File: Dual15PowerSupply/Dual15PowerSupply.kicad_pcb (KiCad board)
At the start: 2 copper layers, 100 x 100 mm, 37 parts, among them J1 120VAC, J2 +/-15VDC, U1 LT3091, U2 LT3081

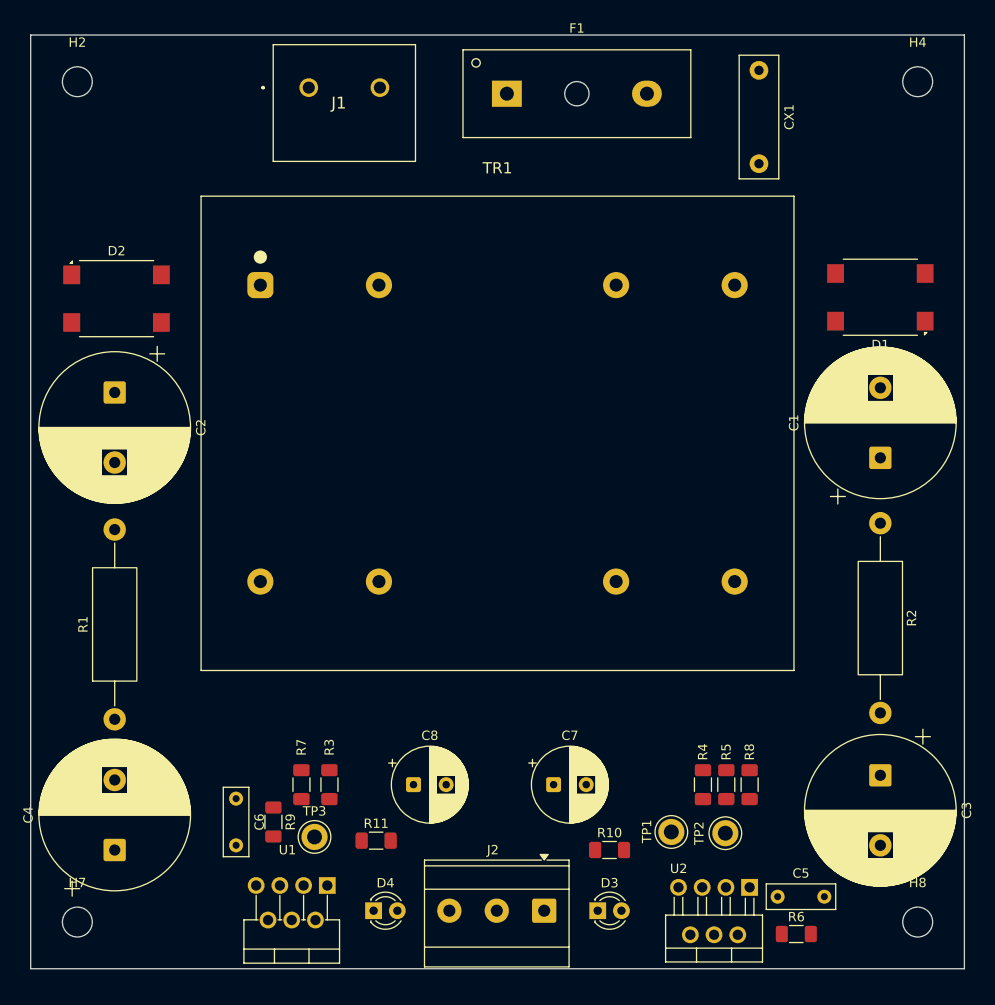
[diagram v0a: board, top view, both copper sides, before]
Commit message: Layout in progress
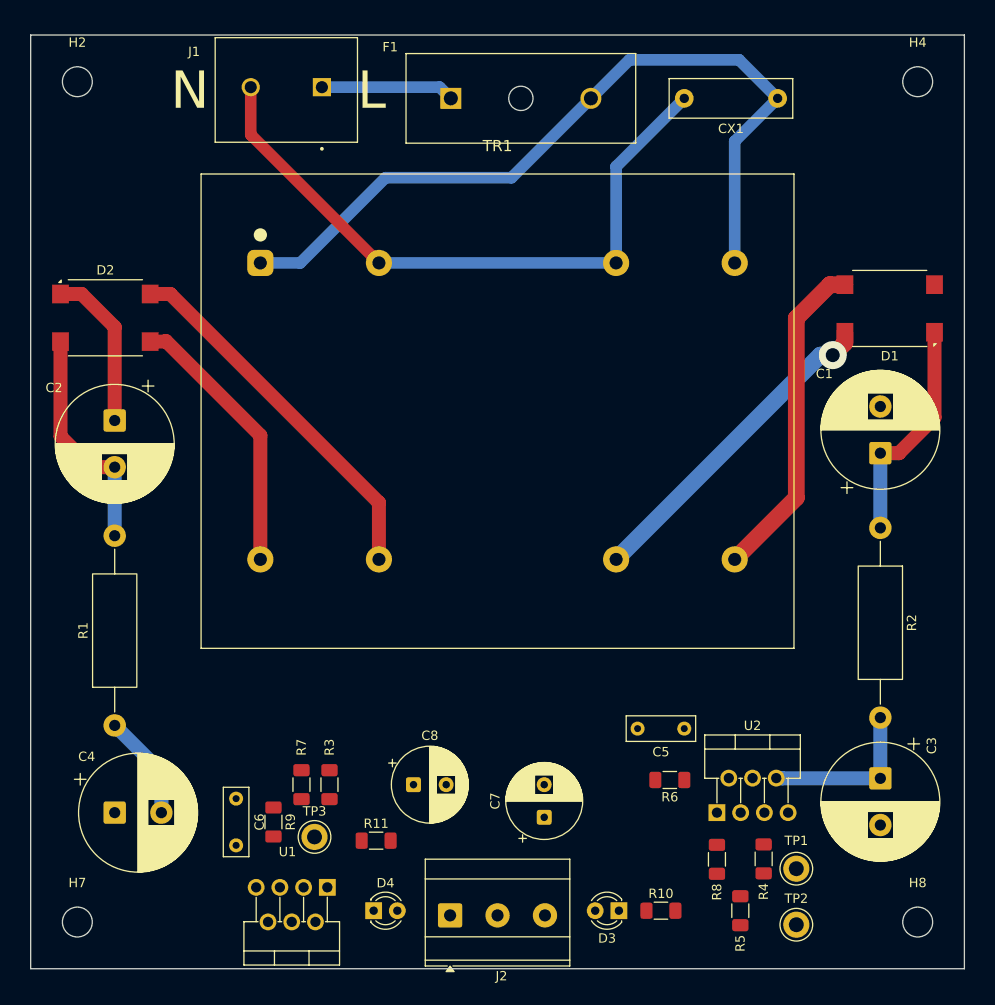
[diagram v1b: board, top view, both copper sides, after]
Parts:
- C1, C2: value 2200µF -> 1000µF; footprint Capacitor_THT:CP_Radial_D16.0mm_P7.50mm -> Capacitor_THT:CP_Radial_D12.5mm_P5.00mm
- C3, C4: footprint Capacitor_THT:CP_Radial_D16.0mm_P7.50mm -> Capacitor_THT:CP_Radial_D12.5mm_P5.00mm
- F1: footprint Fuseholder_Wurth:Wurth_WR-FSH_696105003002 -> Fuseholder_Wurth_WR-FSH:J_Wurth_WR-FSH_696105003002
- J1: footprint TerminalBlock_762:MKDS 5_2-7,62 -> TerminalBlock_Phoenix:PHOENIX_1731721
- U2: footprint Package_TO_SOT_THT:TO-220-7_P2.54x5.08mm_StaggerOdd_Lead3.08mm_Vertical -> Package_TO_SOT_THT:TO-220-7_P2.54x3.7mm_StaggerOdd_Lead3.8mm_Vertical
- moved R6 21.4 mm to (168.4, 111.5), turned to 180 degrees
- moved C5 20.6 mm to (170.0, 106.0), turned to 180 degrees
- moved TP1 14.0 mm to (182.0, 121.0)
- moved R5 13.6 mm to (176.0, 125.5), turned to -90 degrees
- moved F1 13.5 mm to (145.0, 38.5)
- moved TP2 12.4 mm to (182.0, 127.0), turned to -90 degrees
- moved R4 10.3 mm to (178.5, 120.0), turned to -90 degrees
- moved J2 10.1 mm to (144.9, 126.0), turned to 0 degrees
- moved R8 8.73 mm to (173.5, 120.0), turned to 90 degrees
- moved U2 8.73 mm to (173.5, 115.0), turned to 0 degrees
- moved R10 8.51 mm to (167.5, 125.5)
- moved J1 7.47 mm to (135.0, 32.0), turned to 180 degrees
- moved C4 4.00 mm to (109.0, 115.0), turned to 0 degrees
- moved C7 3.64 mm to (155.0, 115.5), turned to 90 degrees
- moved CX1 3.61 mm to (180.0, 38.5), turned to 180 degrees
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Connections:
- net Net-(D1-+) renamed /RawDC+
- net Net-(D1-Pad3) renamed /S1
- net Net-(D1-Pad4) renamed /S2
- net Net-(D2--) renamed /RawDC-
- net Net-(D2-Pad3) renamed /S4
- net Net-(D2-Pad4) renamed /S3
- J1 pad 1: /AC_N -> /AC_L
- J1 pad 2: /AC_L -> /AC_N
- J2 pad 1: /+15VDC -> /-15VDC
- J2 pad 3: /-15VDC -> /+15VDC
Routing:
- net /AC_L_Fused: track 0.00 -> 85.6 mm
- net /AC_N: track 0.00 -> 70.6 mm
- net /S3: track 0.00 -> 39.8 mm
- net /S1: track 0.00 -> 35.2 mm
- net /S2: track 0.00 -> 35.2 mm, vias 0 -> 1
- net /S4: track 0.00 -> 29.3 mm
- net /RawDC-: track 0.00 -> 24.7 mm
- net /RawDC+: track 0.00 -> 24.5 mm
- net GND: track 0.00 -> 17.3 mm
- net /Vin+: track 0.00 -> 17.1 mm
- net /AC_L: track 0.00 -> 14.3 mm
- net /Vin-: track 0.00 -> 11.4 mm
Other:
- board text added: "L"
- board text added: "N"
